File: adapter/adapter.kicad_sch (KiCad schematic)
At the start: 20 parts, among them J10 Ribbon, J11 Ribbon, J12 Ribbon, J3 battery charge, J6 battery charge, J7 trackball, J8 trackball, J9 Ribbon, SW1 SW_SPST, SW2 SW_SPST, SW3 SW_SPST, SW4 SW_SPST, U1 eliteC, U2 eliteC

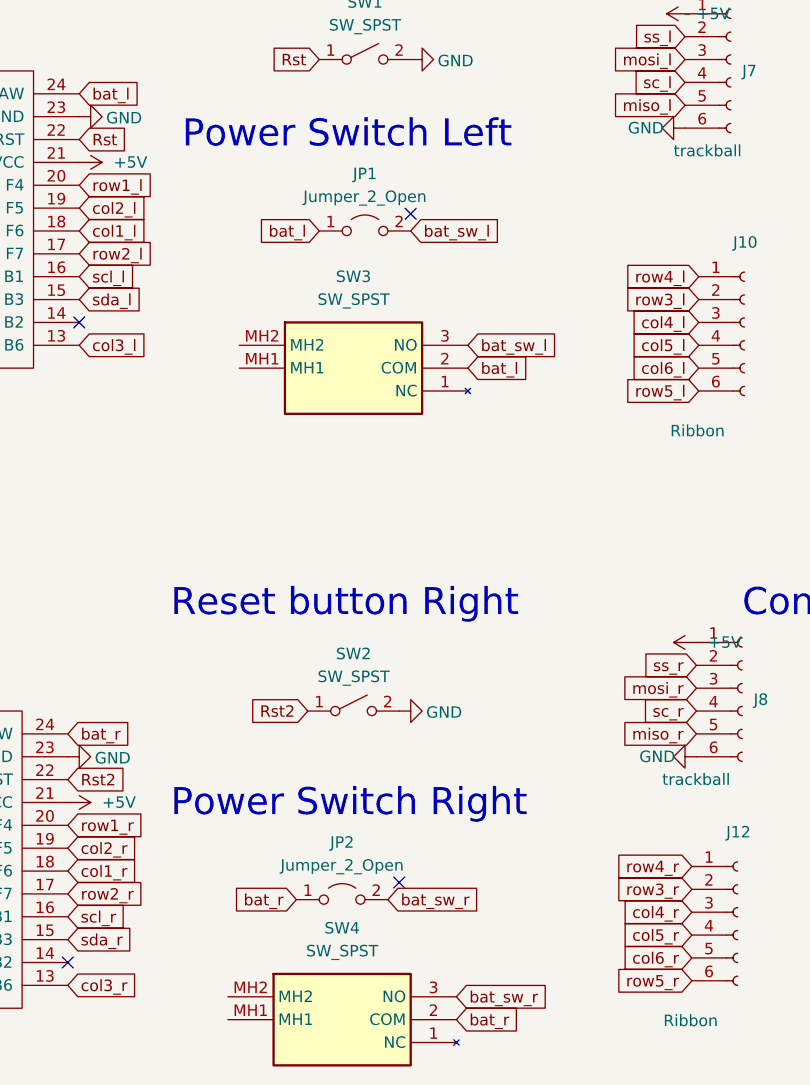
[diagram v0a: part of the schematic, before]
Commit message: simplify
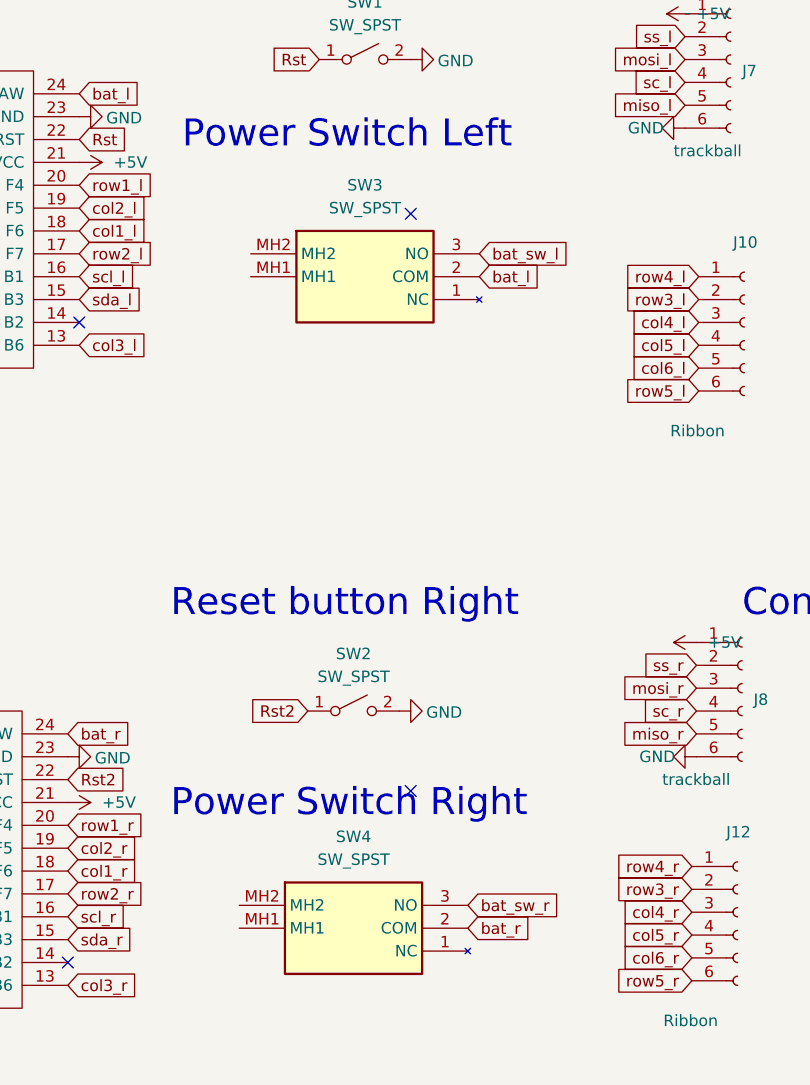
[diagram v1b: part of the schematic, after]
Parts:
- removed JP1, JP2: Jumper_2_Open, Library:power_switch_jumper, symbol Jumper:Jumper_2_Open
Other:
- moved on the sheet: SW3, SW4
